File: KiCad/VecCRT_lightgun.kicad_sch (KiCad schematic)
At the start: 6 parts, among them J8 Conn_01x03, K1 SchEin, Q7 2N7000, X1 OPL820-OC

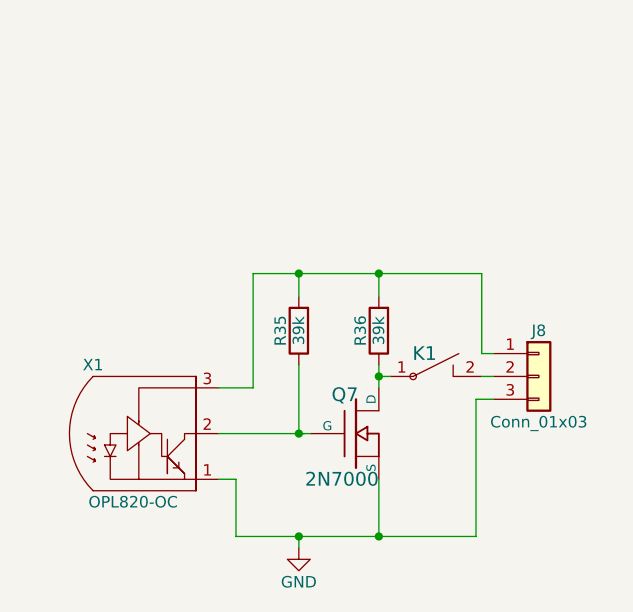
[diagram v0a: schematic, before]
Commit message: lightgun lamp
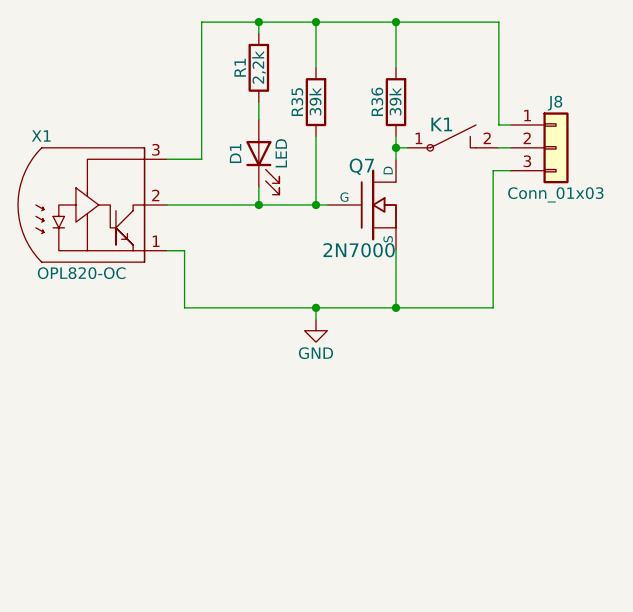
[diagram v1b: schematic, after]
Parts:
- added D1: LED, symbol Device:LED
- added R1: 2,2k, RG:R4-2, symbol Device:R
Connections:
- net at Q7.G, R35.1, X1.2: now also D1.1 (K)
- net at J8.1 (Pin_1), R35.2, R36.2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: now also R1.2
- new net: D1.2 (A), R1.1
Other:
- moved on the sheet: J8, K1, Q7, R35, R36, X1
